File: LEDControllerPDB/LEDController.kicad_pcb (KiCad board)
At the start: 2 copper layers, 104 x 79.1 mm, 33 parts, among them J1 3557-2, J10 3557-2, J11 TB002-500-04BE, J12 TB002-500-04BE, J17 TB002-500-04BE, J2 3557-2, J3 3557-2, J4 3557-2, J5 3557-2, J6 3557-2, J7 0389690002, J9 Conn_01x03_Pin, K1 J115F11CH5VDCS61.5U, M2.5 / #6 MountingHole_2.7mm_M2.5, Q1 DMP3099L, Q3 MMBT2222A

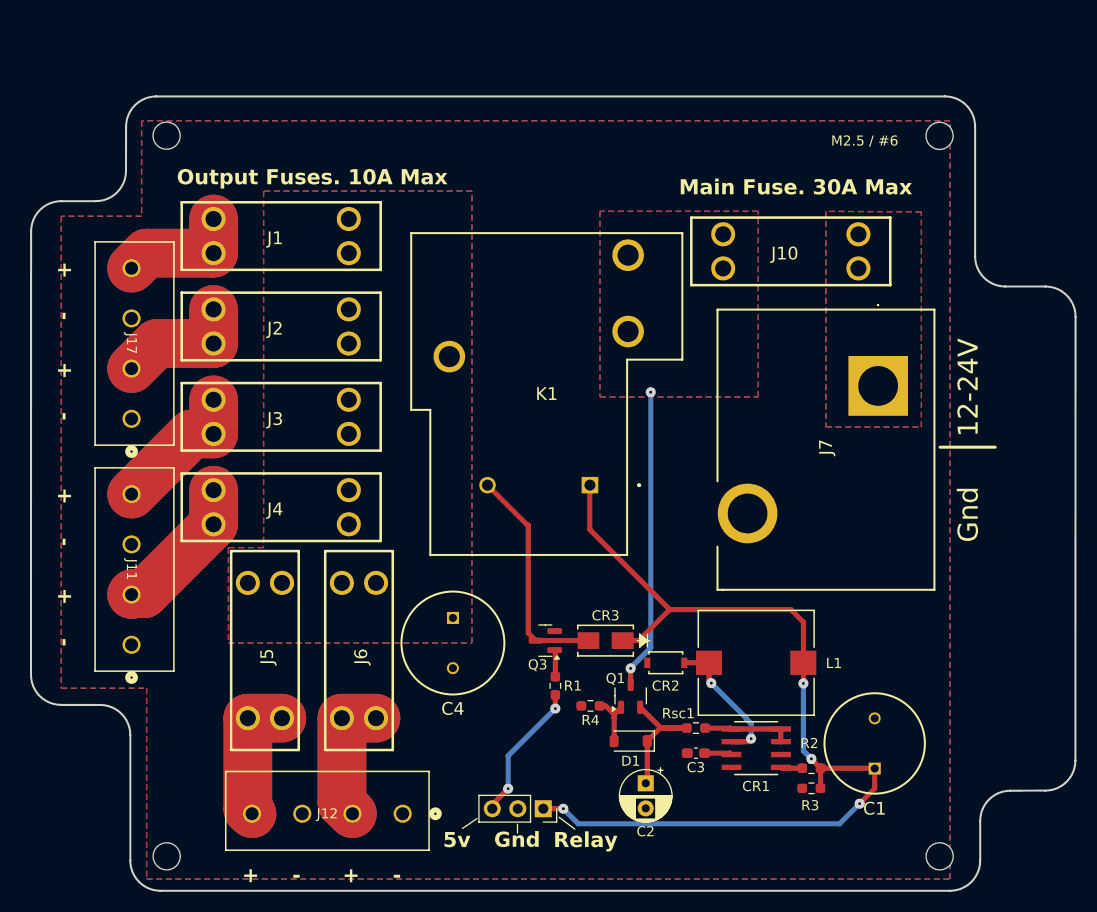
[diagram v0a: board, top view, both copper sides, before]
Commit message: done
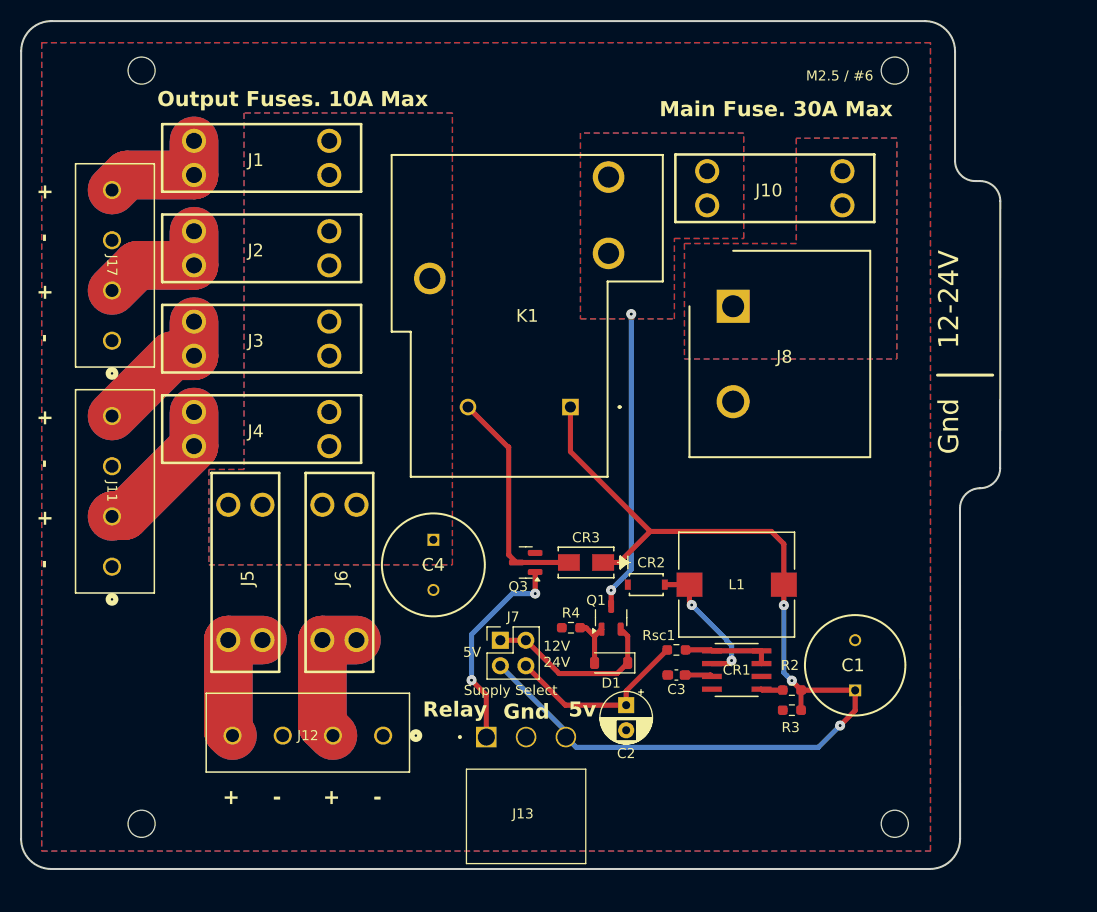
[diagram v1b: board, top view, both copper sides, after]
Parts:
- removed J9: Conn_01x03_Pin, Connector_PinSocket_2.54mm:PinSocket_1x03_P2.54mm_Vertical
- removed R1: 1K, Resistor_SMD:R_0603_1608Metric_Pad0.98x0.95mm_HandSolder
- added J13: 647676-3, LEDController:TE_647676-3, F.Cu at (83.8, 102.9)
- added J8: HB9500-9.5-2P, LEDController:SHDR2W140P0X950_1X2_2055X1800X1440P, F.Cu at (108.4, 60.0)
- J7: value 0389690002 -> Conn_02x02_Row_Letter_First; footprint LEDController:0389690002 -> Connector_PinHeader_2.54mm:PinHeader_2x02_P2.54mm_Vertical
- moved J7 45.4 mm to (85.2, 93.2), turned to 0 degrees
- moved J3 8.02 mm to (61.5, 63.2)
- moved C2 8.02 mm to (97.8, 99.7)
- moved C3 8.02 mm to (102.8, 96.7)
- moved CR1 8.02 mm to (108.8, 96.2)
- moved CR2 8.02 mm to (99.8, 87.7)
- moved CR3 8.02 mm to (93.8, 85.5)
- moved D1 8.02 mm to (96.3, 95.5)
- moved L1 8.02 mm to (108.8, 87.7)
- moved Q1 8.02 mm to (96.3, 91.0)
- moved Q3 8.02 mm to (87.8, 85.5)
- moved R2 8.02 mm to (114.3, 98.2)
- moved R3 8.02 mm to (114.3, 100.2)
- moved R4 8.02 mm to (92.3, 92.0)
- moved Rsc1 8.02 mm to (102.8, 94.2)
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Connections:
- D1 pad 1: /5VReg/Vin -> Net-(D1-K)
- J7 pad 1: /50U -> Net-(D1-K)
- J7 pad 2: GND -> Net-(D1-K)
- Q1 pad 2: /5VReg/Vin -> Net-(D1-K)
- Q3 pad 1: Net-(Q3-B) -> /Relay Controll
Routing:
- net /Relay Controll: track 0.00 -> 21.1 mm, vias 0 -> 2
- net Net-(D1-K): track 0.00 -> 18.1 mm
- net Net-(J9-Pin_3): track 13.9 -> 0.00 mm, vias 2 -> 0
- net /5V: track 95.2 -> 100.7 mm, vias 4 -> 3
- net /5VReg/Vin: track 14.2 -> 19.0 mm
- net Net-(Q3-B): track 2.66 -> 0.00 mm
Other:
- board size 104 x 79.1 mm -> 97.5 x 84.4 mm
- board text added: "12V 24V"
- board text added: "5V"
- board text added: "Supply Select"
